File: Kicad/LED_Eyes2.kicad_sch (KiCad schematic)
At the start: 44 parts, among them J2 Conn_01x03, U202 74LVC1G17

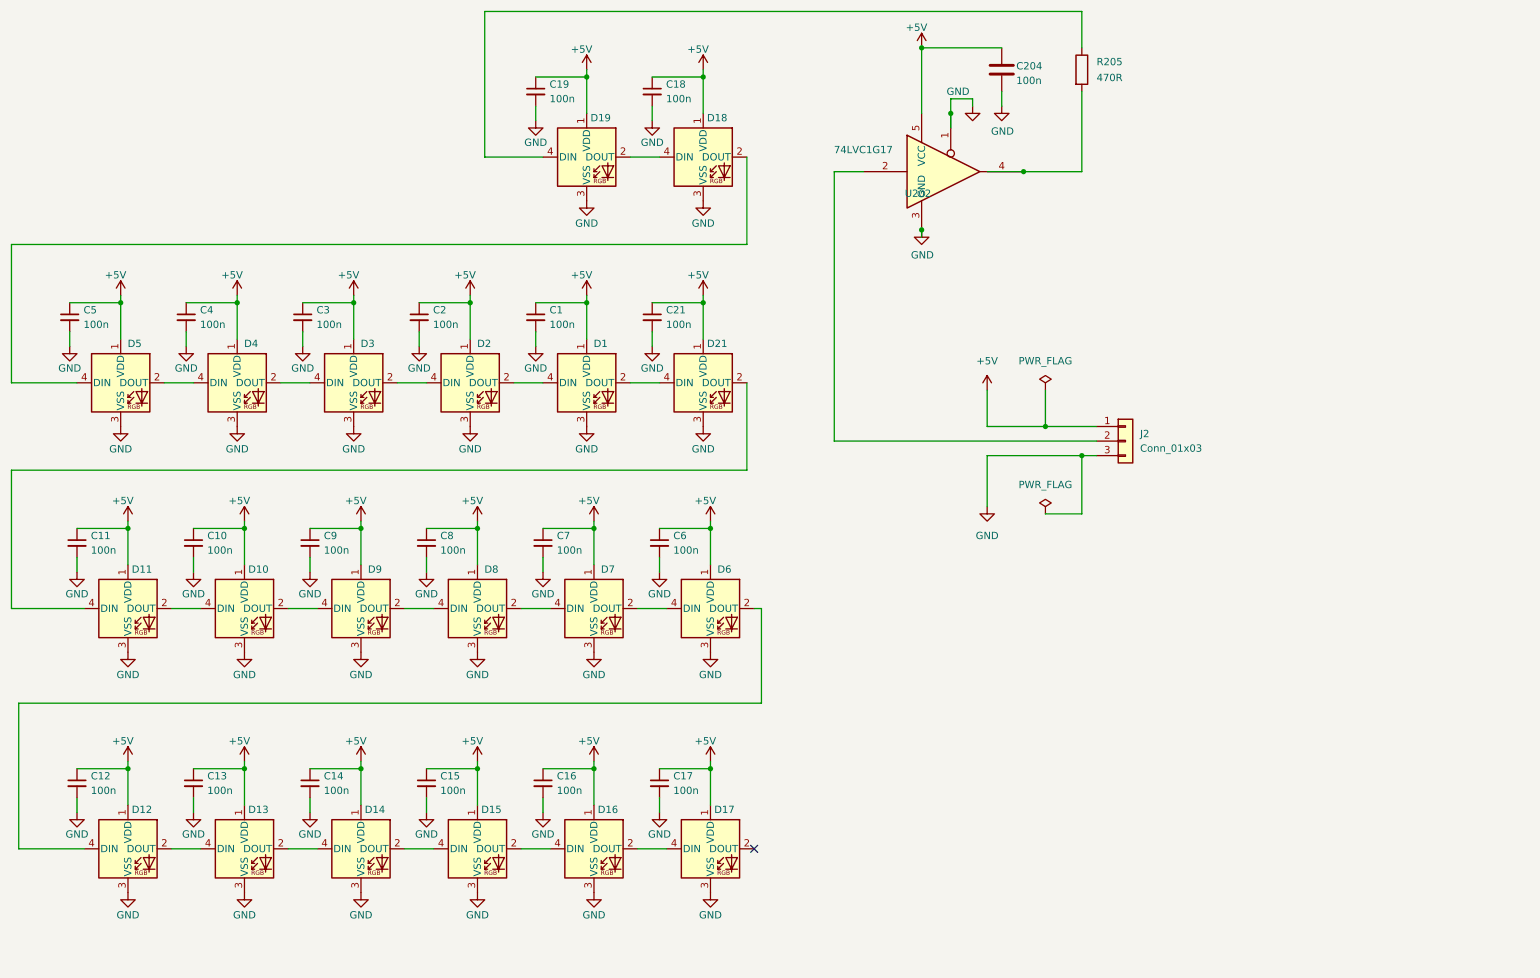
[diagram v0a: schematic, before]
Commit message: PCB_Layout sketched
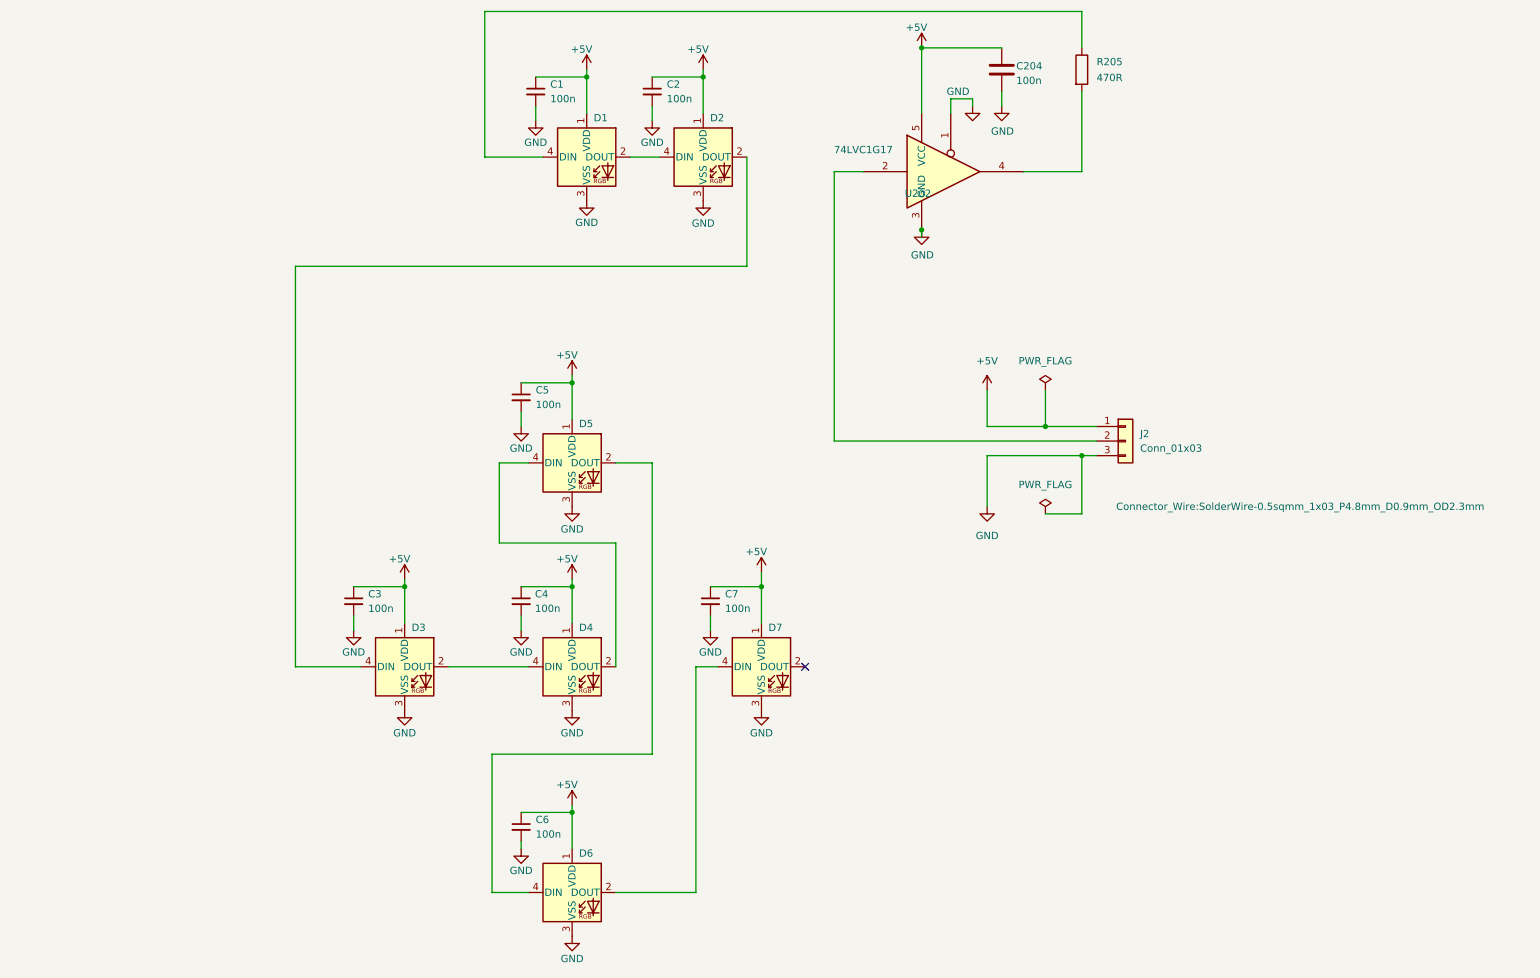
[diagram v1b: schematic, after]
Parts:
- removed C1, C10, C11, C12, C13, C14, C15, C16, C17, C6, C7, C8, C9: 100n, Capacitor_SMD:C_0805_2012Metric_Pad1.18x1.45mm_HandSolder, symbol Device:C_Small
- removed D1, D10, D11, D12, D13, D14, D15, D16, D17, D6, D7, D8, D9: WS2812B, LED_SMD:LED_WS2812B_PLCC4_5.0x5.0mm_P3.2mm, symbol LED:WS2812B
- J2: footprint (none) -> Connector_Wire:SolderWire-0.5sqmm_1x03_P4.8mm_D0.9mm_OD2.3mm
- renumbered C19 to C1, C18 to C2, C5 to C3, C3 to C5, C2 to C6, C21 to C7, D19 to D1, D18 to D2, D5 to D3, D3 to D5, D2 to D6, D21 to D7
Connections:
- net at D6.2 (DOUT): now also D7.4 (DIN)
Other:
- moved on the sheet: C3, C4, C5, C6, C7, D3, D4, D5, D6, D7
